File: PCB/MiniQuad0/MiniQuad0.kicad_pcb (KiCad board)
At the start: 2 copper layers, 36 x 50 mm, 30 parts, among them J1 R8EF_Radio, J10 BMP280_breakout, J11 HMC5883L_breakout, J12 MAG_drdy, J13 BAR_CSB, J14 BAR_SD0, J15 MCU_BOOT, J16 MCU_RST, J17 MCU_SWDIO, J2 POWER, J3 ESC_A, J4 ESC_B, J5 ESC_C, J6 ESC_D, J7 POWER, J8 VBAT, J9 RADIO_SIG, Q1 2N2222, U1 LSM6DSOTR, U2 XIAO-RP2350-SMD

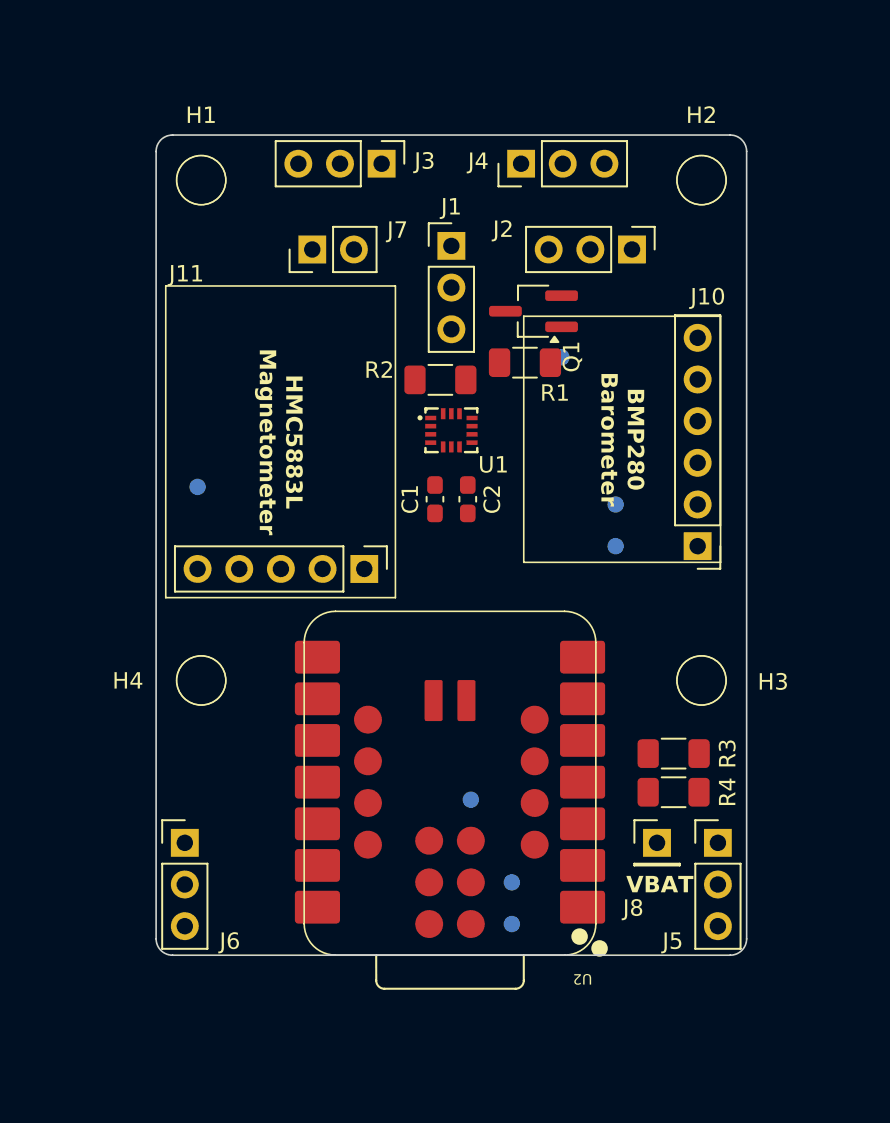
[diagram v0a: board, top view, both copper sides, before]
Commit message: changed pin defs, finished PCB
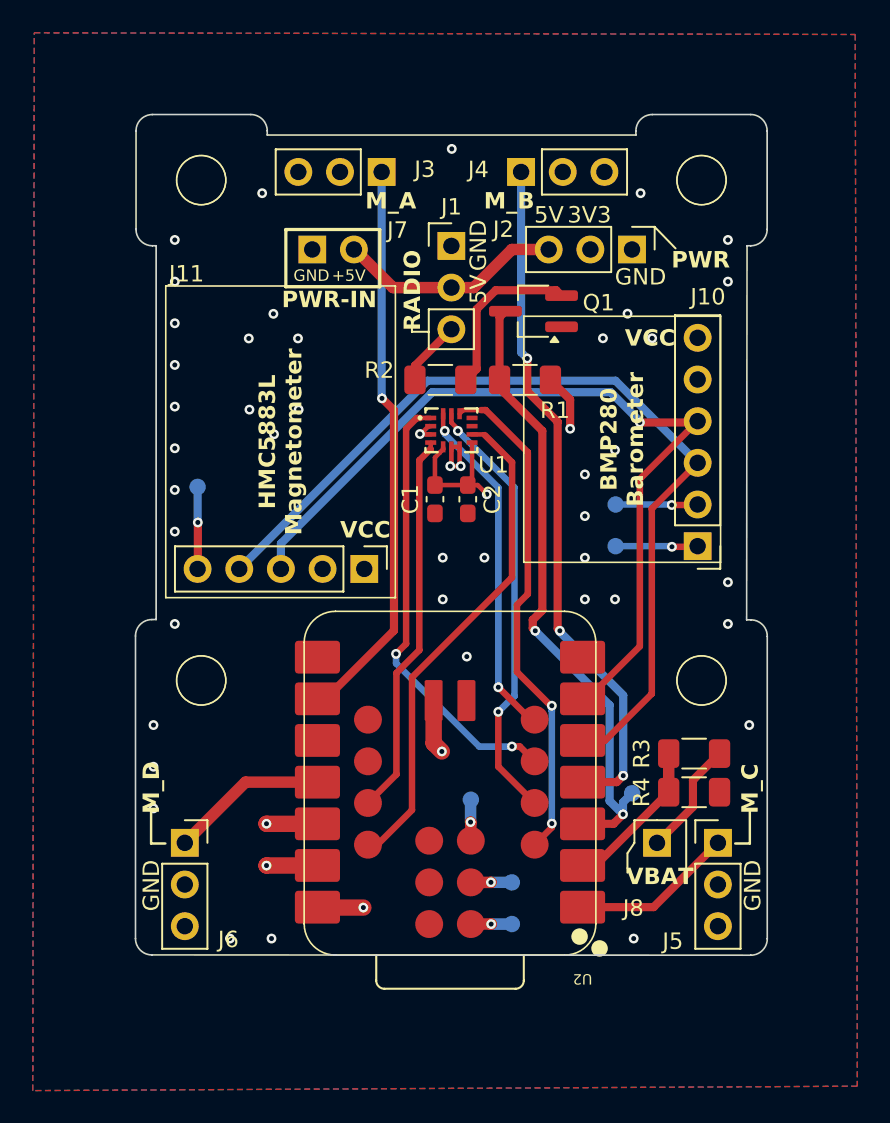
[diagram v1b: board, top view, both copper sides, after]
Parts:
- moved J9 26.9 mm to (159.0, 127.1)
- moved R3 1.25 mm to (162.8, 124.7)
- moved R4 1.25 mm to (162.8, 127.1)
- moved R1 1.05 mm to (152.5, 101.9)
- moved J3 0.50 mm to (143.8, 89.2)
- moved J4 0.50 mm to (152.2, 89.2)
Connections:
- U2 pad 1: /BAT_SENSE -> /MOTOR_C
- U2 pad 10: /IMU_SD0 -> unconnected-(U2-GPIO4/D9/SPI0_MISO-Pad10)
- U2 pad 11: /IMU_SDA -> /MOTOR_D
- U2 pad 15: unconnected-(U2-GPIO21/D11/RX1-Pad15) -> /IMU_INT2
- U2 pad 16: unconnected-(U2-GPIO20/D12/TX1-Pad16) -> /IMU_INT1
- U2 pad 17: /IMU_I2C_SCL -> unconnected-(U2-GPIO17/D13/SCL0-Pad17)
- U2 pad 18: /IMU_I2C_SDA -> unconnected-(U2-GPIO16/D14/SDA0-Pad18)
- U2 pad 19: unconnected-(U2-GPIO11/D15/SPI1_MOSI-Pad19) -> /IMU_SDA
- U2 pad 2: /MOTOR_A -> /BAT_SENSE
- U2 pad 20: /IMU_INT1 -> /IMU_SD0
- U2 pad 21: /IMU_INT2 -> /IMU_SCL
- U2 pad 22: /RADIO_SIG -> /IMU_CS
- U2 pad 3: /MOTOR_B -> /RADIO_SIG
- U2 pad 4: /MOTOR_C -> /MOTOR_B
- U2 pad 5: /MOTOR_D -> /IMU_I2C_SDA
- U2 pad 6: /IMU_SD0 -> /IMU_I2C_SCL
- U2 pad 9: /IMU_SCL -> /MOTOR_A
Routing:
- net +5V: track 0.00 -> 59.9 mm, vias 0 -> 1
- net /IMU_I2C_SDA: track 0.00 -> 55.4 mm
- net /IMU_I2C_SCL: track 0.00 -> 51.6 mm, vias 0 -> 1
- net /MOTOR_B: track 0.00 -> 42.0 mm, vias 0 -> 3
- net /RADIO_SIG: track 0.00 -> 38.6 mm, vias 0 -> 2
- net /MOTOR_A: track 0.00 -> 34.7 mm, vias 0 -> 1
- net /IMU_CS: track 0.00 -> 30.9 mm, vias 0 -> 2
- net /IMU_INT2: track 0.00 -> 30.4 mm
- net /IMU_SD0: track 0.00 -> 27.3 mm, vias 0 -> 2
- net /IMU_SCL: track 0.00 -> 26.7 mm, vias 0 -> 2
- net /IMU_INT1: track 0.00 -> 23.6 mm
- net /IMU_SDA: track 0.00 -> 21.1 mm, vias 0 -> 2
- net +3.3V: track 0.00 -> 16.7 mm, vias 0 -> 4
- net Net-(Q1-B): track 0.00 -> 10.4 mm
- net GND: track 0.00 -> 9.97 mm, vias 0 -> 46
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- added copper zone on In2.Cu, net +3.3V
- added copper zone on B.Cu, net GND
- added copper zone on F.Cu, net GND
- added copper zone on In1.Cu, net GND
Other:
- board size 36 x 50 mm -> 38.5 x 51.2 mm
- copper layers 2 -> 4
- board text added: "+5V"
- board text added: "3V3"
- board text added: "5V"
- board text added: "GND"
- board text added: "M_A"
- board text added: "M_B"
- board text added: "M_C"
- board text added: "M_D"
- board text added: "PWR"
- board text added: "PWR-IN"
- board text added: "RADIO"
- board text added: "VCC"
